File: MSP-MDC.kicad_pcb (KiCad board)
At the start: 2 copper layers, 104.1 x 106.7 mm, 40 parts, among them U10 74LS00, U11 74LS32, U12 74LS86, U13 74LS166, U14 74LS374, U15 74LS138, U16 74LS257, U17 74LS257, U18 74LS257, U19 74LS257, U2 Z80CPU, U20 74LS283, U3 74LS374, U4 74ALS00, U5 74ALS32, U6 74LS245, U7 74ALS244, U8 74LS283

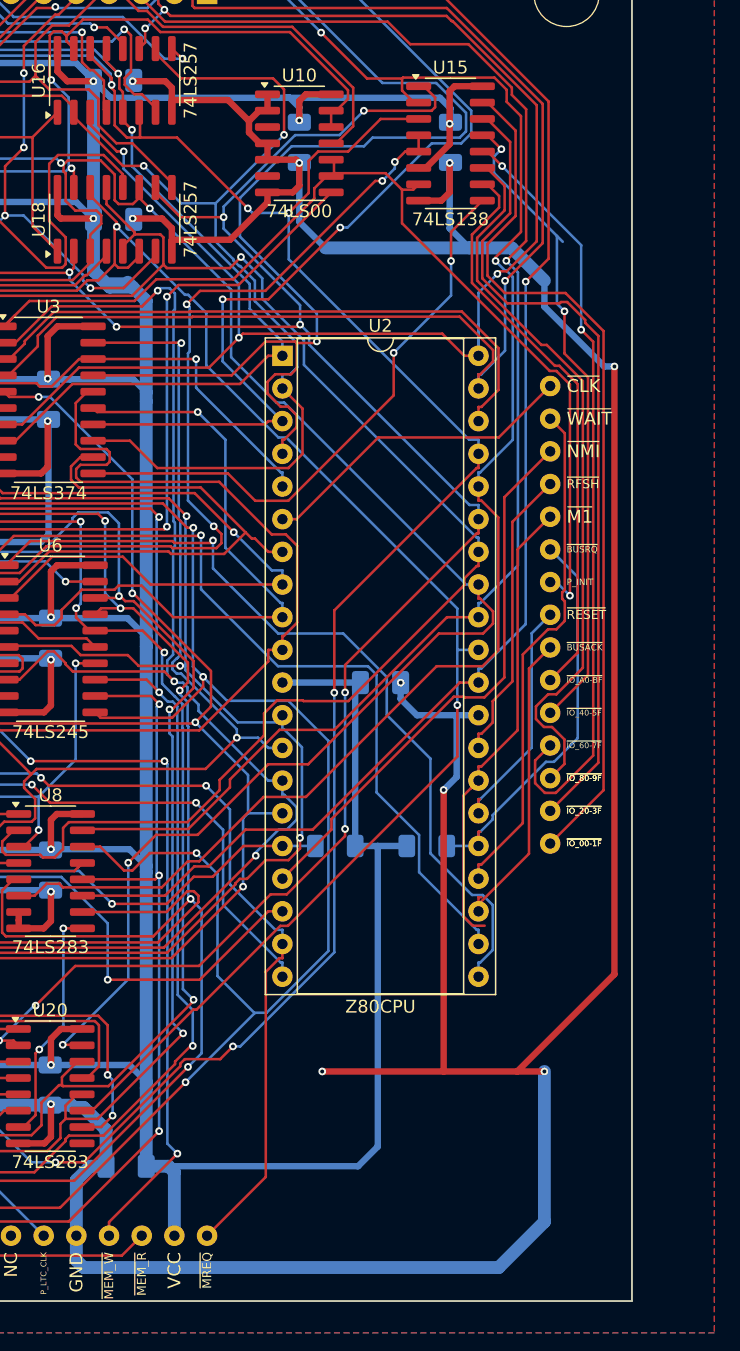
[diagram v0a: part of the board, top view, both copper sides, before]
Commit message: Resize the board
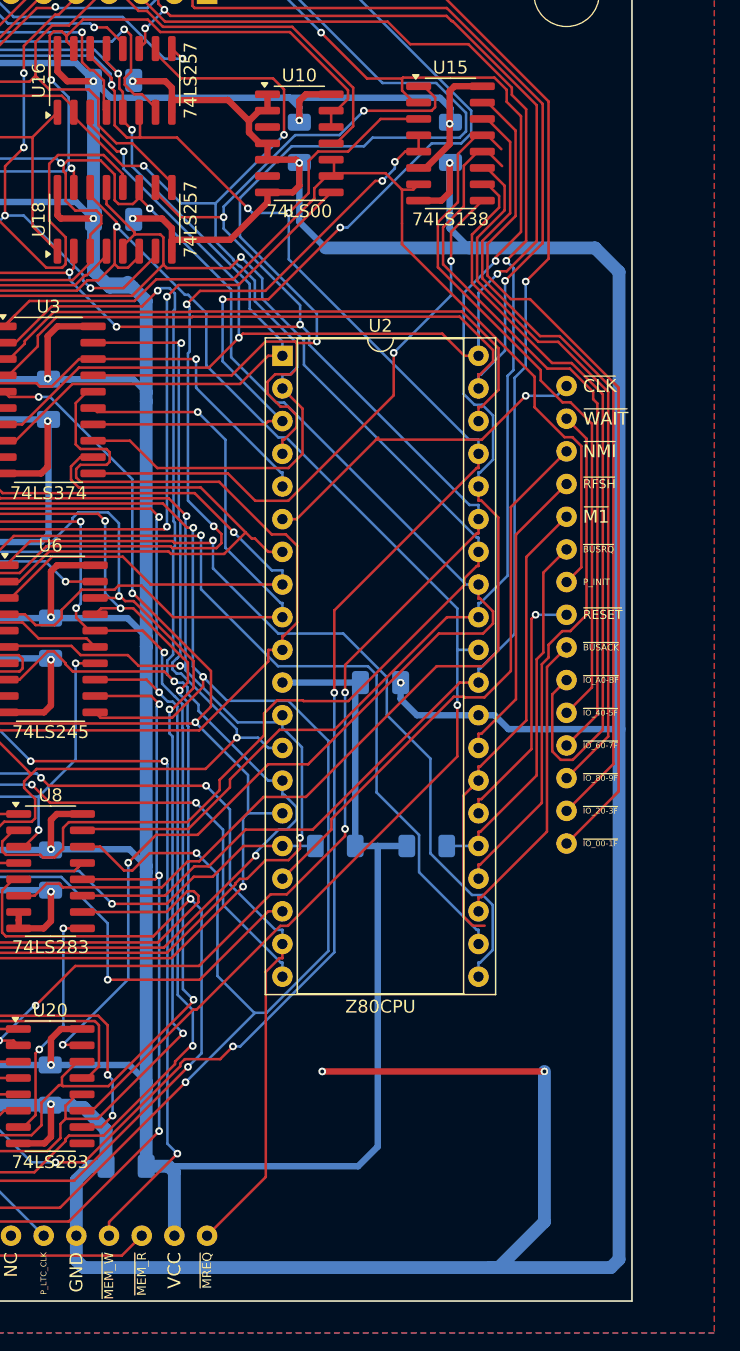
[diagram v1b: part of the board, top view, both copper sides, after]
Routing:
- net /J1-24: track 44.7 -> 60.3 mm
- net GND: track 819.4 -> 827.8 mm, vias 30 -> 28
- net /J1-21: track 50.9 -> 54.6 mm, vias 2 -> 0
- net /J1-22: track 60.2 -> 56.6 mm, vias 2 -> 0
- net /J1-16: track 31.8 -> 28.4 mm
- net /J1-1: track 79.9 -> 77.8 mm, vias 1 -> 0
- net /J1-20: track 63.9 -> 62.4 mm
- net /J3-20: track 25.1 -> 26.6 mm, vias 0 -> 1
- net /J1-19: track 68.0 -> 66.6 mm
- net /J1-8: track 114.6 -> 113.8 mm
- net /J1-23: track 56.5 -> 55.7 mm
- net /Top Board/A4: track 147.4 -> 146.8 mm
- net /J1-11: track 126.5 -> 126.0 mm
- net /Top Board/A5: track 175.7 -> 175.2 mm
- net /Top Board/A7: track 186.7 -> 186.2 mm
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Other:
- board text removed: "~{IO_00-1F}"
- board text removed: "~{IO_20-3F}"
- board text removed: "~{IO_80-9F}"
